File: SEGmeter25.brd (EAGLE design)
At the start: 114.3 x 87.6 mm, 137 parts, among them IC1 DS1307, IC2 LD1117S50, IC3 LD1117S33, IC4 XBEE, IC5 ATmega328, IC6 MCP1541, IC7 MCP3208, J1 Short 12V, J10 3.5mm, J11 3.5mm, J12 3.5mm, J13 3.5mm, J14 Relays, J15 3.5mm, J16 Star ground, J17 3.5mm, J18 Arduino-compatible headers, J19 3.5mm, J2 1-Wire, J20 3.5mm, J3 ISP, J4 Power, J5 Comms, J6 MICROSD, J7 Buttons, J8 Relay LEDs, J9 Sensor 5V, Q1 32768 Hz, Q2 16 MHz, Q3 2N7002, Q4 2N7002, Q5 2N7002

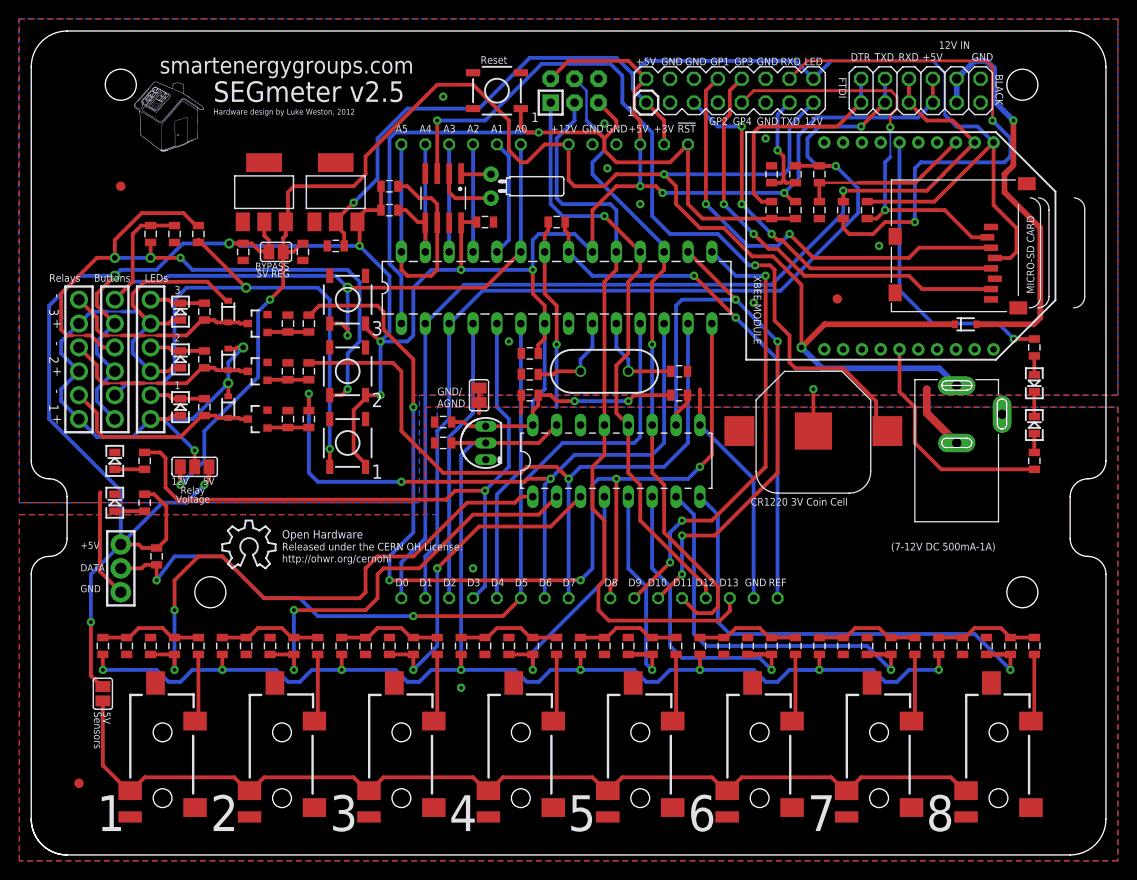
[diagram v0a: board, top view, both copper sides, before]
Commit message: foo
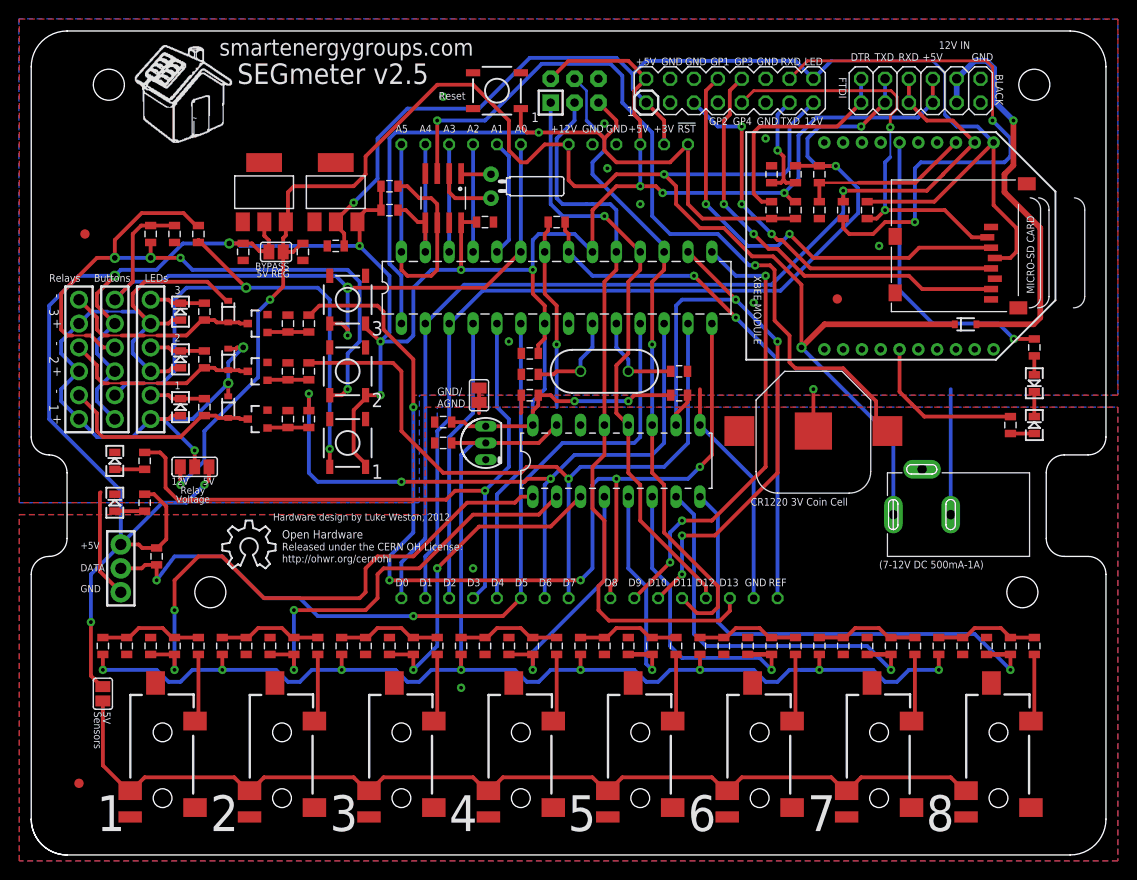
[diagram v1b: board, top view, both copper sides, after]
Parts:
- moved J4 7.65 mm to (92.7, 34.3), turned to 90 degrees
- moved FID3 6.35 mm to (0.64, 64.1)
- moved R8 4.58 mm to (99.1, 43.8), turned to 270 degrees
- moved H2 1.27 mm to (3.17, 80.0)
- moved H3 1.27 mm to (101.6, 80.0)
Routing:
- net N$5: track 24.5 -> 17.4 mm
- net +12V: track 181.2 -> 184.8 mm
- net GND: track 57.3 -> 56.6 mm
- net N$6: track 2.01 -> 2.54 mm
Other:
- outline, holes or cut-outs redrawn
